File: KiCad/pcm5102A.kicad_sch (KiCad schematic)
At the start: 18 parts, among them J19 positivePowerInputs, U10 PCM5102APW

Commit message: Changes to the BoM
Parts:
- C12, C13: Part_Number (none) -> GRM155R71H222KA01D
- C14, C23: Part_Number (none) -> GRM188R71A225KE15D
- C15, C16, C17, C18: Part_Number (none) -> C0603C104K5RACTU
- C19, C20, C21, C22: Part_Number (none) -> UWT1H100MCL1GB
- J19: Part_Number (none) -> SSK02-FPH-254-A3
- R11, R12: Part_Number (none) -> RK73H2BTTD4700F
- R18: Part_Number (none) -> CRCW040222R0FKED
- U10: Part_Number (none) -> PCM5102APW
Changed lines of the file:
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@@
 			)
 		)
-		(property "Datasheet" ""
+		(property "Datasheet" "https://www.koaspeer.com/pdfs/RK73H.pdf"
 			(at 92.71 57.15 0)
 			(hide yes)
@@
 		(property "Description" "Resistor, US symbol"
 			(at 92.71 57.15 0)
+			(hide yes)
+			(show_name no)
+			(do_not_autoplace no)
+			(effects
+				(font
+					(size 1.27 1.27)
+				)
+			)
+		)
+		(property "Part_Number" "RK73H2BTTD4700F"
+			(at 92.71 57.15 90)
 			(hide yes)
 			(show_name no)
@@
 			)
 		)
-		(property "Datasheet" ""
+		(property "Datasheet" "https://www.digikey.com/en/products/detail/same-sky-formerly-cui-devices/SSK02-FPH-254-A3/28772125"
 			(at 71.12 35.56 0)
 			(hide yes)
@@
 				)
 				(justify bottom)
+			)
+		)
+		(property "Part_Number" "SSK02-FPH-254-A3"
+			(at 71.12 35.56 90)
+			(hide yes)
+			(show_name no)
+			(do_not_autoplace no)
+			(effects
+				(font
+					(size 1.27 1.27)
+				)
 			)
 		)
@@
 			)
 		)
-		(property "Datasheet" ""
+		(property "Datasheet" "https://www.digikey.com/en/products/detail/kemet/C0603C104K5RACTU/1465594"
 			(at 181.61 60.96 0)
 			(hide yes)
@@
 		)
 		(property "Description" "Unpolarized capacitor, small symbol"
+			(at 181.61 60.96 0)
+			(hide yes)
+			(show_name no)
+			(do_not_autoplace no)
+			(effects
+				(font
+					(size 1.27 1.27)
+				)
+			)
+		)
+		(property "Part_Number" "C0603C104K5RACTU"
 			(at 181.61 60.96 0)
 			(hide yes)
@@
 			)
 		)
+		(property "Part_Number" ""
+			(at 179.07 77.47 0)
+			(hide yes)
+			(show_name no)
+			(do_not_autoplace no)
+			(effects
+				(font
+					(size 1.27 1.27)
+				)
+			)
+		)
 		(pin "1"
 		)
@@
 			)
 		)
-		(property "Datasheet" ""
+		(property "Datasheet" "https://www.digikey.com/en/products/detail/murata-electronics/GRM188R71A225KE15D/1033256?s=N4IgTCBcDaIOICUCyBGAHGhB2FBBMYArANICiKhAIiALoC%2BQA"
 			(at 128.27 87.63 0)
 			(hide yes)
@@
 		)
 		(property "Description" "Unpolarized capacitor, small symbol"
+			(at 128.27 87.63 0)
+			(hide yes)
+			(show_name no)
+			(do_not_autoplace no)
+			(effects
+				(font
+					(size 1.27 1.27)
+				)
+			)
+		)
+		(property "Part_Number" "GRM188R71A225KE15D"
 			(at 128.27 87.63 0)
 			(hide yes)
@@
 			)
 		)
-		(property "Datasheet" ""
+		(property "Datasheet" "https://www.digikey.com/en/products/detail/murata-electronics/GRM155R71H222KA01D/587234?s=N4IgTCBcDaIOICUCyBGArGhB2FAJMBA0gIIAMKAIiALoC%2BQA"
 			(at 99.06 63.5 0)
 			(hide yes)
@@
 		)
 		(property "Description" "Unpolarized capacitor, small symbol"
+			(at 99.06 63.5 0)
+			(hide yes)
+			(show_name no)
+			(do_not_autoplace no)
+			(effects
+				(font
+					(size 1.27 1.27)
+				)
+			)
+		)
+		(property "Part_Number" "GRM155R71H222KA01D"
 			(at 99.06 63.5 0)
 			(hide yes)
@@
 			)
 		)
+		(property "Part_Number" "PCM5102APW"
+			(at 148.59 71.12 0)
+			(hide yes)
+			(show_name no)
+			(do_not_autoplace no)
+			(effects
+				(font
+					(size 1.27 1.27)
+				)
+			)
+		)
 		(pin "4"
 		)
@@
 			)
 		)
-		(property "Datasheet" "https://www.nichicon.co.jp/english/series_items/catalog_pdf/e-ucq.pdf"
+		(property "Datasheet" "https://www.nichicon.co.jp/english/series_items/catalog_pdf/e-uwt.pdf"
 			(at 224.79 55.88 0)
 			(hide yes)
@@
 		)
 		(property "Description" "Polarized capacitor, small US symbol"
+			(at 224.79 55.88 0)
+			(hide yes)
+			(show_name no)
+			(do_not_autoplace no)
+			(effects
+				(font
+					(size 1.27 1.27)
+				)
+			)
+		)
+		(property "Part_Number" "UWT1H100MCL1GB"
 			(at 224.79 55.88 0)
 			(hide yes)
@@
 			)
 		)
-		(property "Datasheet" ""
+		(property "Datasheet" "https://www.digikey.com/en/products/detail/kemet/C0603C104K5RACTU/1465594"
 			(at 214.63 55.88 0)
 			(hide yes)
@@
 		)
 		(property "Description" "Unpolarized capacitor, small symbol"
+			(at 214.63 55.88 0)
+			(hide yes)
+			(show_name no)
+			(do_not_autoplace no)
+			(effects
+				(font
+					(size 1.27 1.27)
+				)
+			)
+		)
+		(property "Part_Number" "C0603C104K5RACTU"
 			(at 214.63 55.88 0)
 			(hide yes)
@@
 			)
 		)
-		(property "Datasheet" ""
+		(property "Datasheet" "https://www.digikey.com/en/products/detail/kemet/C0603C104K5RACTU/1465594"
 			(at 232.41 50.8 0)
 			(hide yes)
@@
 		)
 		(property "Description" "Unpolarized capacitor, small symbol"
+			(at 232.41 50.8 0)
+			(hide yes)
+			(show_name no)
+			(do_not_autoplace no)
+			(effects
+				(font
+					(size 1.27 1.27)
+				)
+			)
+		)
+		(property "Part_Number" "C0603C104K5RACTU"
 			(at 232.41 50.8 0)
 			(hide yes)
@@
 			)
 		)
-		(property "Datasheet" ""
+		(property "Datasheet" "https://www.digikey.com/en/products/detail/vishay-dale/CRCW040222R0FKED/1177815"
 			(at 172.72 66.04 0)
 			(hide yes)
@@
 		(property "Description" "Resistor, small US symbol"
 			(at 172.72 66.04 0)
+			(hide yes)
+			(show_name no)
+			(do_not_autoplace no)
+			(effects
+				(font
+					(size 1.27 1.27)
+				)
+			)
+		)
+		(property "Part_Number" "CRCW040222R0FKED"
+			(at 172.72 66.04 90)
 			(hide yes)
 			(show_name no)
@@
 			)
 		)
-		(property "Datasheet" ""
+		(property "Datasheet" "https://www.digikey.com/en/products/detail/murata-electronics/GRM155R71H222KA01D/587234?s=N4IgTCBcDaIOICUCyBGArGhB2FAJMBA0gIIAMKAIiALoC%2BQA"
 			(at 80.01 63.5 0)
 			(hide yes)
@@
 		)
 		(property "Description" "Unpolarized capacitor, small symbol"
+			(at 80.01 63.5 0)
+			(hide yes)
+			(show_name no)
+			(do_not_autoplace no)
+			(effects
+				(font
+					(size 1.27 1.27)
+				)
+			)
+		)
+		(property "Part_Number" "GRM155R71H222KA01D"
 			(at 80.01 63.5 0)
 			(hide yes)
@@
 			)
 		)
-		(property "Datasheet" ""
+		(property "Datasheet" "https://www.digikey.com/en/products/detail/murata-electronics/GRM188R71A225KE15D/1033256?s=N4IgTCBcDaIOICUCyBGAHGhB2FBBMYArANICiKhAIiALoC%2BQA"
 			(at 125.73 72.39 0)
 			(hide yes)
@@
 		)
 		(property "Description" "Unpolarized capacitor, small symbol"
+			(at 125.73 72.39 0)
+			(hide yes)
+			(show_name no)
+			(do_not_autoplace no)
+			(effects
+				(font
+					(size 1.27 1.27)
+				)
+			)
+		)
+		(property "Part_Number" "GRM188R71A225KE15D"
 			(at 125.73 72.39 0)
 			(hide yes)
@@
 			)
 		)
-		(property "Datasheet" ""
+		(property "Datasheet" "https://www.koaspeer.com/pdfs/RK73H.pdf"
 			(at 105.41 60.96 0)
 			(hide yes)
@@
 		(property "Description" "Resistor, US symbol"
 			(at 105.41 60.96 0)
+			(hide yes)
+			(show_name no)
+			(do_not_autoplace no)
+			(effects
+				(font
+					(size 1.27 1.27)
+				)
+			)
+		)
+		(property "Part_Number" "RK73H2BTTD4700F"
+			(at 105.41 60.96 90)
 			(hide yes)
 			(show_name no)
@@
 			)
 		)
-		(property "Datasheet" "https://www.nichicon.co.jp/english/series_items/catalog_pdf/e-ucq.pdf"
+		(property "Datasheet" "https://www.nichicon.co.jp/english/series_items/catalog_pdf/e-uwt.pdf"
 			(at 242.57 50.8 0)
 			(hide yes)
@@
 		)
 		(property "Description" "Polarized capacitor, small US symbol"
+			(at 242.57 50.8 0)
+			(hide yes)
+			(show_name no)
+			(do_not_autoplace no)
+			(effects
+				(font
+					(size 1.27 1.27)
+				)
+			)
+		)
+		(property "Part_Number" "UWT1H100MCL1GB"
 			(at 242.57 50.8 0)
 			(hide yes)
@@
 			)
 		)
-		(property "Datasheet" "https://www.nichicon.co.jp/english/series_items/catalog_pdf/e-ucq.pdf"
+		(property "Datasheet" "https://www.nichicon.co.jp/english/series_items/catalog_pdf/e-uwt.pdf"
 			(at 191.77 60.96 0)
 			(hide yes)
@@
 		)
 		(property "Description" "Polarized capacitor, small US symbol"
+			(at 191.77 60.96 0)
+			(hide yes)
+			(show_name no)
+			(do_not_autoplace no)
+			(effects
+				(font
+					(size 1.27 1.27)
+				)
+			)
+		)
+		(property "Part_Number" "UWT1H100MCL1GB"
 			(at 191.77 60.96 0)
 			(hide yes)
@@
 			)
 		)
-		(property "Datasheet" "https://www.nichicon.co.jp/english/series_items/catalog_pdf/e-ucq.pdf"
+		(property "Datasheet" "https://www.nichicon.co.jp/english/series_items/catalog_pdf/e-uwt.pdf"
 			(at 110.49 50.8 0)
 			(hide yes)
@@
 		)
 		(property "Description" "Polarized capacitor, small US symbol"
+			(at 110.49 50.8 0)
+			(hide yes)
+			(show_name no)
+			(do_not_autoplace no)
+			(effects
+				(font
+					(size 1.27 1.27)
+				)
+			)
+		)
+		(property "Part_Number" "UWT1H100MCL1GB"
 			(at 110.49 50.8 0)
 			(hide yes)
@@
 			)
 		)
-		(property "Datasheet" ""
+		(property "Datasheet" "https://www.digikey.com/en/products/detail/kemet/C0603C104K5RACTU/1465594"
 			(at 120.65 50.8 0)
 			(hide yes)
@@
 			(at 120.65 50.8 0)
 			(hide yes)
+			(show_name no)
+			(do_not_autoplace no)
+			(effects
+				(font
+					(size 1.27 1.27)
+				)
+			)
+		)
+		(property "Part_Number" "C0603C104K5RACTU"
+			(at 120.65 50.8 0)
+			(hide yes)

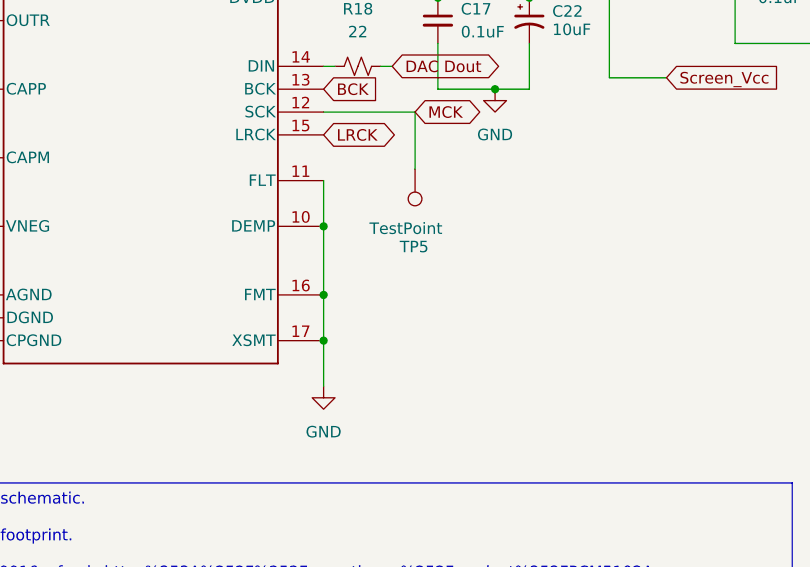
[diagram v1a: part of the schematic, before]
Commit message: done
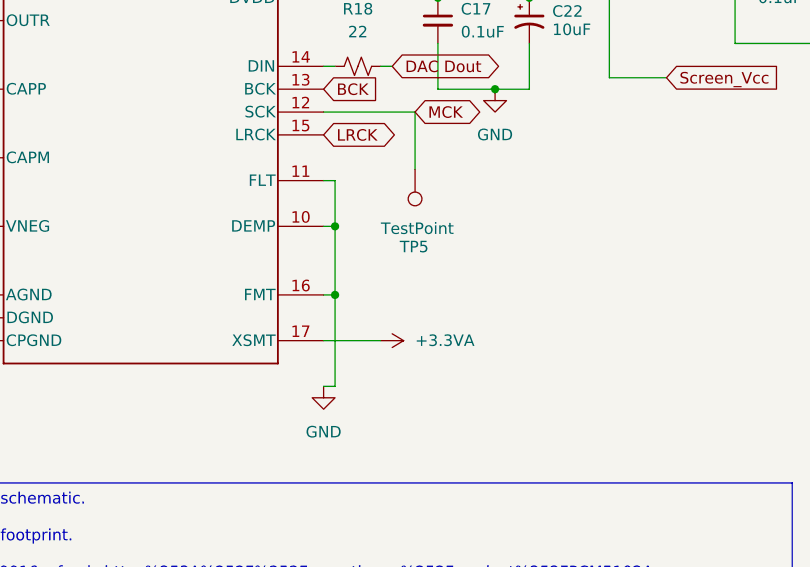
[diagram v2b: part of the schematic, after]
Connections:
- net +3.3VA: now also U10.17 (XSMT)
- net GND: no longer U10.17 (XSMT)
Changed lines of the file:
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@@
-	)
-	(junction
-		(at 168.91 96.52)
-		(diameter 0)
-		(color 0 0 0 0)
 	)
 	(junction
@@
 	)
 	(junction
-		(at 168.91 91.44)
+		(at 170.18 91.44)
 		(diameter 0)
 		(color 0 0 0 0)
@@
 	)
 	(junction
-		(at 168.91 83.82)
+		(at 170.18 83.82)
 		(diameter 0)
 		(color 0 0 0 0)
@@
 	(wire
 		(pts
-			(xy 168.91 83.82) (xy 168.91 91.44)
+			(xy 170.18 78.74) (xy 168.91 78.74)
+		)
+		(stroke
+			(width 0)
+			(type default)
+		)
+	)
+	(wire
+		(pts
+			(xy 170.18 83.82) (xy 170.18 91.44)
 		)
 		(stroke
@@
 	(wire
 		(pts
+			(xy 175.26 96.52) (xy 168.91 96.52)
+		)
+		(stroke
+			(width 0)
+			(type default)
+		)
+	)
+	(wire
+		(pts
 			(xy 179.07 77.47) (xy 179.07 71.12)
 		)
@@
 	(wire
 		(pts
+			(xy 170.18 101.6) (xy 168.91 101.6)
+		)
+		(stroke
+			(width 0)
+			(type default)
+		)
+	)
+	(wire
+		(pts
 			(xy 170.18 66.04) (xy 168.91 66.04)
 		)
@@
 	(wire
 		(pts
-			(xy 168.91 78.74) (xy 168.91 83.82)
+			(xy 170.18 78.74) (xy 170.18 83.82)
 		)
 		(stroke
@@
 	(wire
 		(pts
-			(xy 168.91 91.44) (xy 168.91 96.52)
-		)
-		(stroke
-			(width 0)
-			(type default)
-		)
-	)
-	(wire
-		(pts
 			(xy 187.96 68.58) (xy 191.77 68.58)
 		)
@@
 	(wire
 		(pts
+			(xy 170.18 91.44) (xy 168.91 91.44)
+		)
+		(stroke
+			(width 0)
+			(type default)
+		)
+	)
+	(wire
+		(pts
 			(xy 125.73 68.58) (xy 125.73 69.85)
 		)
@@
 	(wire
 		(pts
-			(xy 168.91 96.52) (xy 168.91 101.6)
+			(xy 170.18 91.44) (xy 170.18 101.6)
 		)
 		(stroke
@@
 		(pts
 			(xy 68.58 45.72) (xy 68.58 57.15)
+		)
+		(stroke
+			(width 0)
+			(type default)
+		)
+	)
+	(wire
+		(pts
+			(xy 170.18 83.82) (xy 168.91 83.82)
 		)
 		(stroke
@@
 		)
 		(property "Value" "TestPoint"
-			(at 182.118 84.074 0)
+			(at 183.388 84.074 0)
 			(show_name no)
 			(do_not_autoplace no)
@@
 					(unit 1)
 				)
+			)
+		)
+	)
+	(symbol
+		(lib_id "power:+3.3VA")
+		(at 175.26 96.52 270)
+		(unit 1)
+		(body_style 1)
+		(exclude_from_sim no)
+		(in_bom yes)
+		(on_board yes)
+		(in_pos_files yes)
+		(dnp no)
+		(fields_autoplaced yes)
+		(property "Reference" "#PWR08"
+			(at 171.45 96.52 0)
+			(hide yes)
+			(show_name no)
+			(do_not_autoplace no)
+			(effects
+				(font
+					(size 1.27 1.27)
+				)
+			)
+		)
+		(property "Value" "+3.3VA"
+			(at 179.07 96.5199 90)
+			(show_name no)
+			(do_not_autoplace no)
+			(effects
+				(font
+					(size 1.27 1.27)
+				)
+				(justify left)
+			)
+		)
+		(property "Footprint" ""
+			(at 175.26 96.52 0)
+			(hide yes)
+			(show_name no)
+			(do_not_autoplace no)
+			(effects
+				(font
+					(size 1.27 1.27)
+				)
+			)
+		)
+		(property "Datasheet" ""
+			(at 175.26 96.52 0)
+			(hide yes)
+			(show_name no)
+			(do_not_autoplace no)
+			(effects
+				(font
+					(size 1.27 1.27)
+				)
+			)
+		)
+		(property "Description" "Power symbol creates a global label with name \"+3.3VA\""
+			(at 175.26 96.52 0)
+			(hide yes)
+			(show_name no)
+			(do_not_autoplace no)
+			(effects
+				(font
+					(size 1.27 1.27)
+				)
+			)
+		)
+		(pin "1"
+		)
+		(instances
+			(project "KiCad"
+				(path "/24850b4e-1ce6-41a1-b1f6-c45749a7c3af/6e6f54ae-c134-44a9-b312-648594db47df"
+					(reference "#PWR08")
+					(unit 1)
+				)
